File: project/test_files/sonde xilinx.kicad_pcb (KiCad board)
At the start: 2 copper layers, 29 parts, among them J1 DB25MALE, J2 DB9MALE, P1 CONN_6, U1 74LS125, U2 74LS125

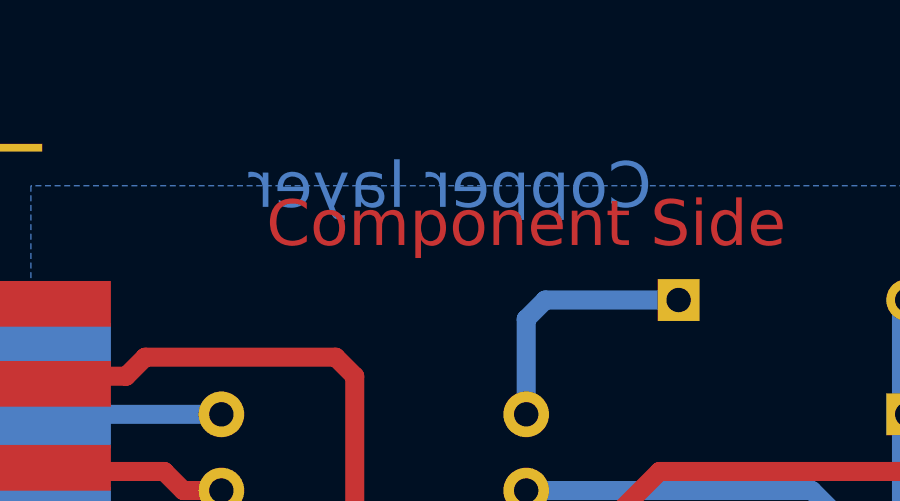
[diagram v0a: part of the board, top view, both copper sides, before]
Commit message: New commit
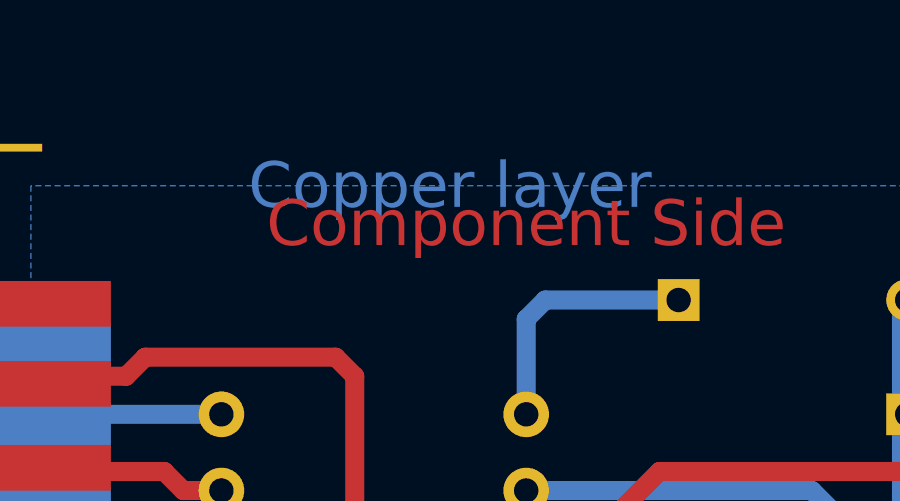
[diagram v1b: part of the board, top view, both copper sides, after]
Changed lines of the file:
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@@
   )
   (gr_text "Copper layer" (at 119.38 68.58) (layer Dessous)
-    (effects (font (size 1.524 1.524) (thickness 0.3048)) (justify mirror))
+    (effects (font (size 1.524 1.524) (thickness 0.3048)))
   )
   (gr_line (start 102.87 110.49) (end 102.87 106.68) (angle 90) (layer Contours.Ci) (width 0.3048))
